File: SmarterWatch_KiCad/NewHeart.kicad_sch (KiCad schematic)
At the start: 1 part, among them U27 BH1792GLC-E2

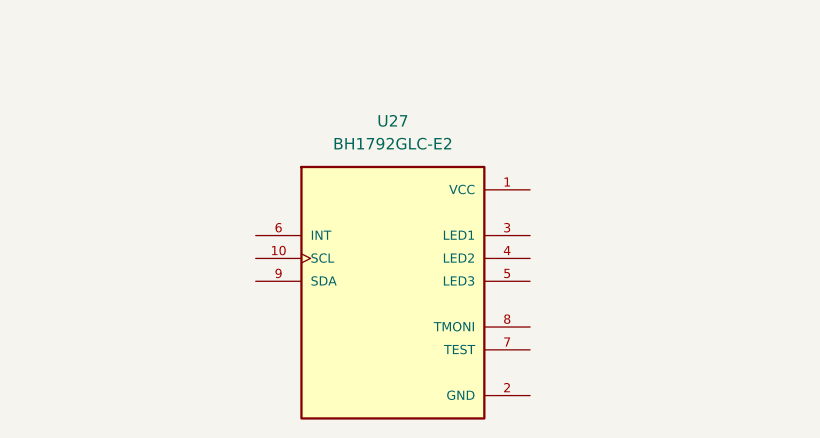
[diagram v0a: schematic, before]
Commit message: Basics of New Heart
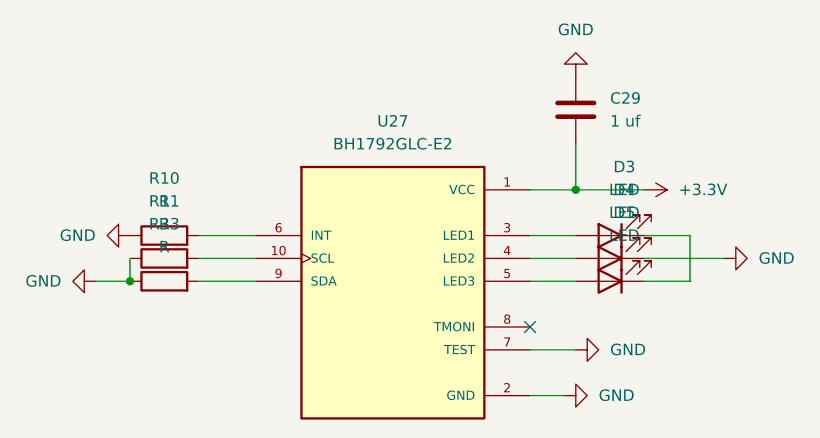
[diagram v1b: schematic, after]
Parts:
- added C29: 1 uf, symbol Device:C
- added D3, D4, D5: LED, symbol Device:LED
- added R10, R11, R33: R, symbol Device:R
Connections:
- net +3.3V: now reaches U27.1 (VCC)
- net +3.3V: now also C29.2
- net at U27.10 (SCL): now also R11.2
- net GND: now reaches U27.2 (GND)
- net GND: now also U27.7 (TEST), C29.1, D4.1 (K), R10.1, R11.1, R33.1
- net at U27.3 (LED1): now also D3.2 (A)
- net at U27.4 (LED2): now also D4.2 (A)
- net at U27.5 (LED3): now also D5.2 (A)
- net at U27.6 (INT): now also R10.2
- net at U27.9 (SDA): now also R33.2
- new net: D3.1 (K), D5.1 (K)
- no-connect marks 0 -> 1
